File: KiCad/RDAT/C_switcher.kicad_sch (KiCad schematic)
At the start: 31 parts, among them J3 USB_C_Receptacle, U5 PTPS25751DREFR

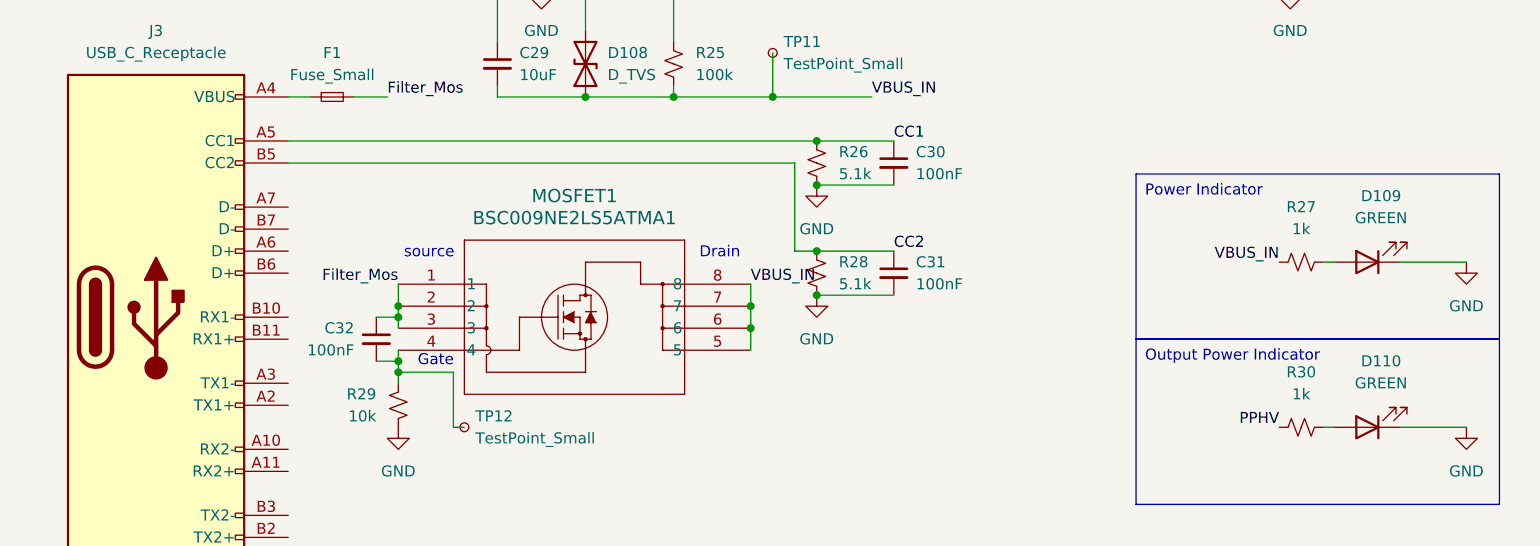
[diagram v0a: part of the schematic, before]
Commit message: added volage stuffs
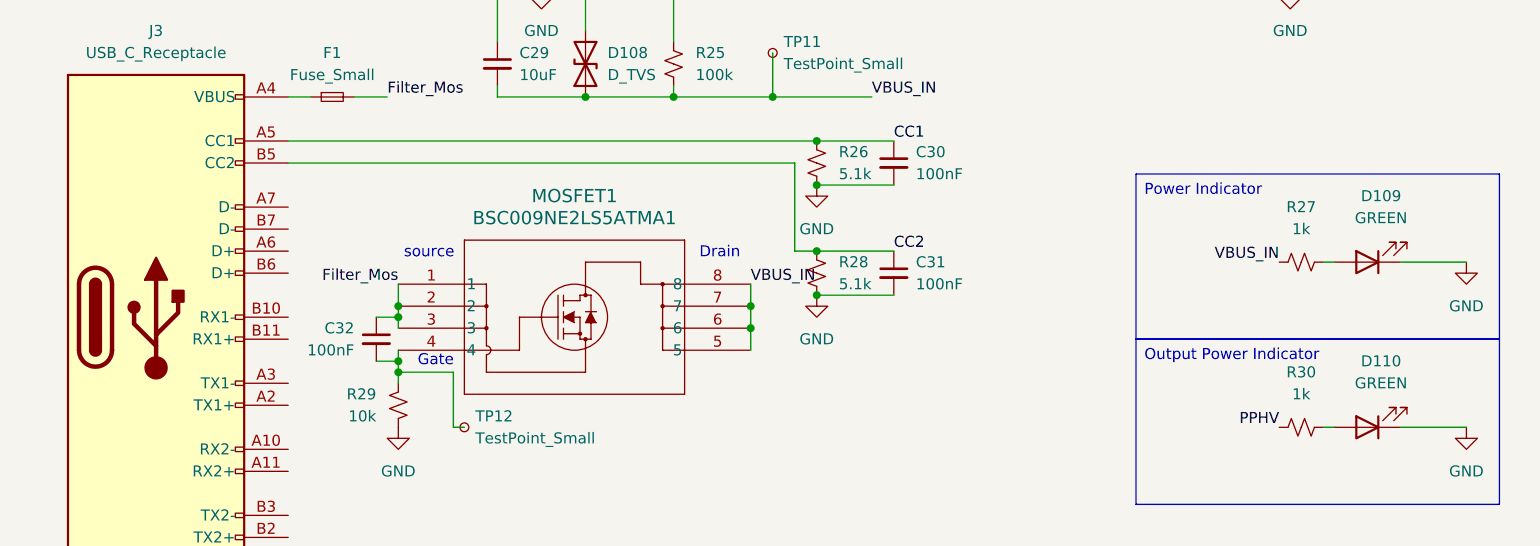
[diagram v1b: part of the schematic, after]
